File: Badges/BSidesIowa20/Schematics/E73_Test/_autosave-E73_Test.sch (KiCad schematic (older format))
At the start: 29 parts, among them J1 Conn_01x02, J2 Oled, J4 Conn_02x04_Odd_Even, J7 USB_C_Receptacle, SW2 SW_DIP_x01, SW4 SW_DIP_x01, U2 TLV1117-33, U3 HX4056, U5 K1-5202UA-03(5Way_Switch)

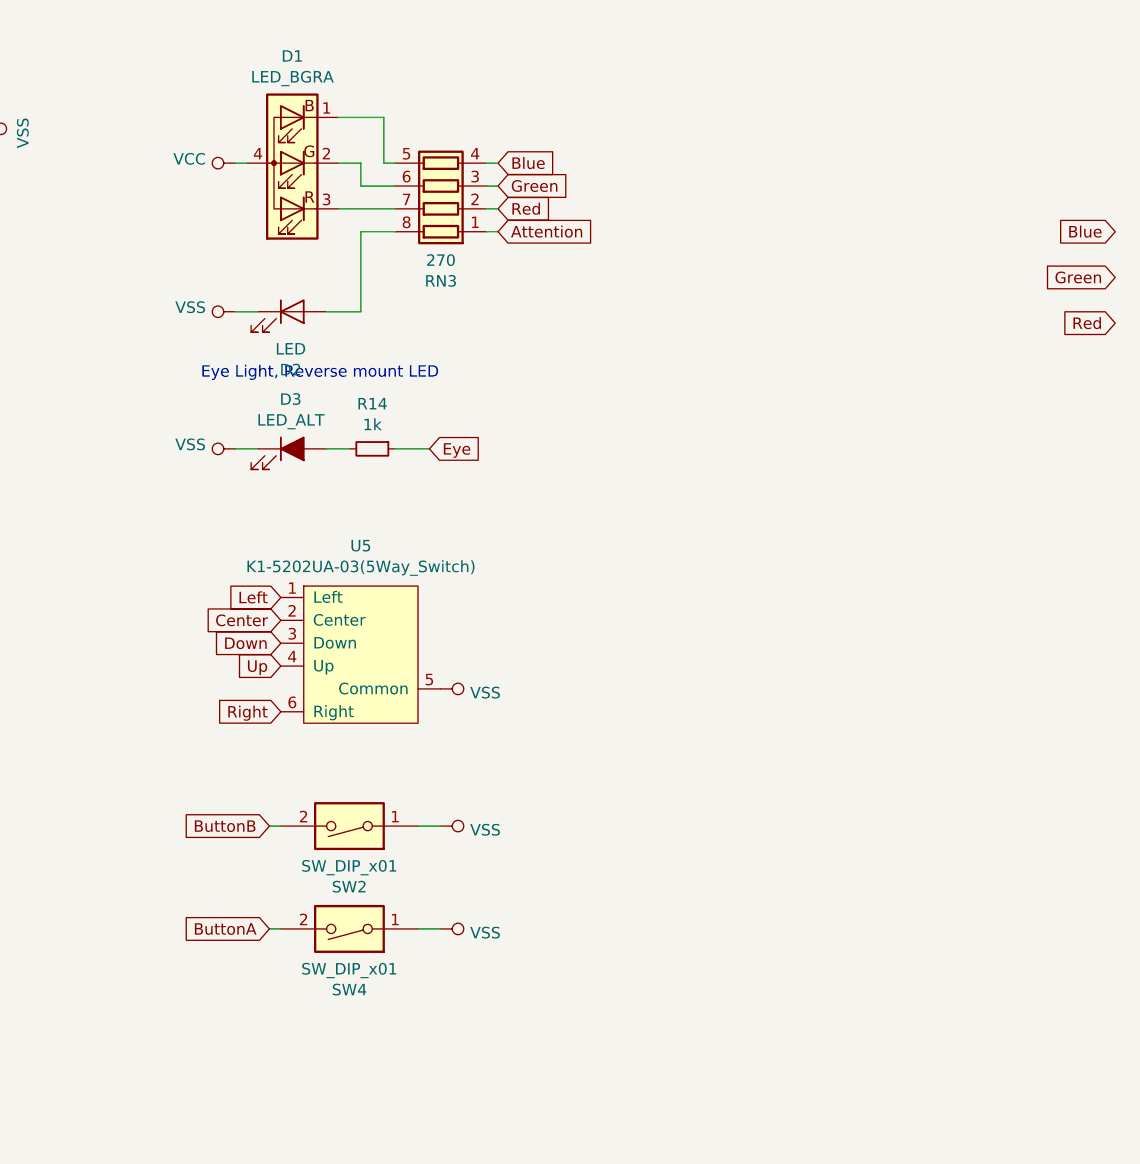
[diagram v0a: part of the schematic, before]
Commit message: Putting stuff together
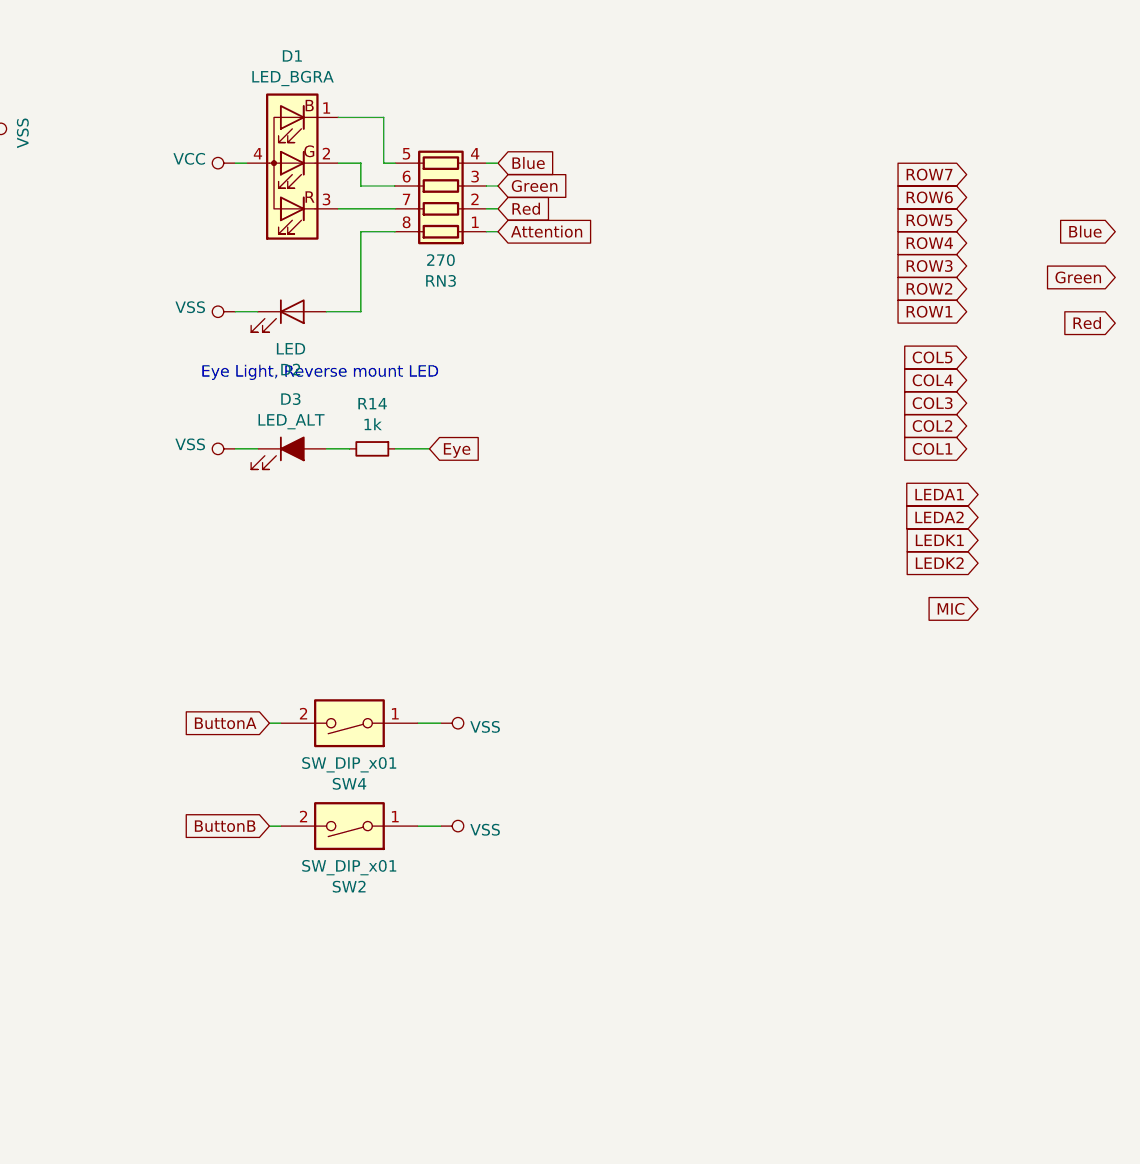
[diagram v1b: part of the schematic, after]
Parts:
- removed U5: K1-5202UA-03(5Way_Switch), Dragos:K1-5202UA-03(5way-switch), symbol dragos-rescue:K1-5202UA-03(5Way_Switch)-Dragos
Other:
- moved on the sheet: SW4
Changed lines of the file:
@@
 Eye Light, Reverse mount LED
-$Comp
-L dragos-rescue:K1-5202UA-03(5Way_Switch)-Dragos U5
-U 1 1 5D705426
-P 4150 3500
-F 0 "U5" H 4150 3975 50  0000 C CNN
-F 1 "K1-5202UA-03(5Way_Switch)" H 4150 3884 50  0000 C CNN
-F 2 "Dragos:K1-5202UA-03(5way-switch)" H 3800 3150 50  0001 C CNN
-F 3 "" H 3800 3150 50  0001 C CNN
-	1    4150 3500
-	1    0    0    -1
-$EndComp
-Text GLabel 3800 3250 0    50   Input ~ 0
-Left
-Text GLabel 3800 3350 0    50   Input ~ 0
-Center
-Text GLabel 3800 3450 0    50   Input ~ 0
-Down
-Text GLabel 3800 3750 0    50   Input ~ 0
-Right
-$Comp
-L power:VSS #PWR0146
-U 1 1 5D7338F5
-P 4500 3650
-F 0 "#PWR0146" H 4500 3500 50  0001 C CNN
-F 1 "VSS" V 4518 3778 50  0000 L CNN
-F 2 "" H 4500 3650 50  0001 C CNN
-F 3 "" H 4500 3650 50  0001 C CNN
-	1    4500 3650
-	0    1    1    0
-$EndComp
 $Comp
 L Switch:SW_DIP_x01 SW2
@@
 Text GLabel 3750 4250 0    50   Input ~ 0
 ButtonB
-Text GLabel 3750 4700 0    50   Input ~ 0
+Text GLabel 3750 3800 0    50   Input ~ 0
 ButtonA
 $Comp
 L Switch:SW_DIP_x01 SW4
 U 1 1 5D7857CD
-P 4100 4700
-F 0 "SW4" H 4100 4967 50  0000 C CNN
-F 1 "SW_DIP_x01" H 4100 4876 50  0000 C CNN
-F 2 "Dragos:1TS002E-2500-2500-CT-HYP-Button" H 4100 4700 50  0001 C CNN
-F 3 "~" H 4100 4700 50  0001 C CNN
-	1    4100 4700
-	-1   0    0    1
-$EndComp
-Wire Wire Line
-	3750 4700 3800 4700
+P 4100 3800
+F 0 "SW4" H 4100 4067 50  0000 C CNN
+F 1 "SW_DIP_x01" H 4100 3976 50  0000 C CNN
+F 2 "Dragos:1TS002E-2500-2500-CT-HYP-Button" H 4100 3800 50  0001 C CNN
+F 3 "~" H 4100 3800 50  0001 C CNN
+	1    4100 3800
+	-1   0    0    1
+$EndComp
+Wire Wire Line
+	3750 3800 3800 3800
 $Comp
 L power:VSS #PWR0148
 U 1 1 5D7857D8
-P 4500 4700
-F 0 "#PWR0148" H 4500 4550 50  0001 C CNN
-F 1 "VSS" V 4518 4828 50  0000 L CNN
-F 2 "" H 4500 4700 50  0001 C CNN
-F 3 "" H 4500 4700 50  0001 C CNN
-	1    4500 4700
-	0    1    1    0
-$EndComp
-Wire Wire Line
-	4500 4700 4400 4700
+P 4500 3800
+F 0 "#PWR0148" H 4500 3650 50  0001 C CNN
+F 1 "VSS" V 4518 3928 50  0000 L CNN
+F 2 "" H 4500 3800 50  0001 C CNN
+F 3 "" H 4500 3800 50  0001 C CNN
+	1    4500 3800
+	0    1    1    0
+$EndComp
+Wire Wire Line
+	4500 3800 4400 3800
 $Comp
 L Device:R_Pack02 RN1
@@
 	0    -1   -1   0
 $EndComp
-Text GLabel 3800 3550 0    50   Input ~ 0
-Up
 $Comp
 L power:+5V #PWR0102
@@
 Text GLabel 9750 5300 0    50   Input ~ 0
 MIC
+Text GLabel 6800 2600 0    50   Input ~ 0
+COL1
+Text GLabel 6800 2500 0    50   Input ~ 0
+COL2
+Text GLabel 6800 2400 0    50   Input ~ 0
+COL3
+Text GLabel 6800 2300 0    50   Input ~ 0
+COL4
+Text GLabel 6800 2200 0    50   Input ~ 0
+COL5
+Text GLabel 6800 2000 0    50   Input ~ 0
+ROW1
+Text GLabel 6800 1900 0    50   Input ~ 0
+ROW2
+Text GLabel 6800 1800 0    50   Input ~ 0
+ROW3
+Text GLabel 6800 1700 0    50   Input ~ 0
+ROW4
+Text GLabel 6800 1600 0    50   Input ~ 0
+ROW5
+Text GLabel 6800 1500 0    50   Input ~ 0
+ROW6
+Text GLabel 6800 1400 0    50   Input ~ 0
+ROW7
+Text GLabel 6850 2800 0    50   Input ~ 0
+LEDA1
+Text GLabel 6850 2900 0    50   Input ~ 0
+LEDA2
+Text GLabel 6850 3000 0    50   Input ~ 0
+LEDK1
+Text GLabel 6850 3100 0    50   Input ~ 0
+LEDK2
+Text GLabel 6850 3300 0    50   Input ~ 0
+MIC
 $EndSCHEMATC
